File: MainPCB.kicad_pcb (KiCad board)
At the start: 4 copper layers, 105 x 62.4 mm, 57 parts, among them J1 RaspberryPi, J2 Conn_01x05, J3 Screw_Terminal_01x02, J4 Conn_01x02, J5 Conn_01x06, J6 Conn_01x03_Pin, J7 Conn_01x05, J8 Conn_01x12, M1 Motor_DC, M2 Motor_DC, M3 Motor_DC, M4 Motor_DC, M5 Motor_DC, SW1 SW_SPDT, SW2 SW_SPDT, SW3 SW_SPDT, SW4 SW_SPDT, U1 Teensy4.1, U10 Compass, U11 V_Regulator5v, U12 RockerSwitch, U13 V_Regulator3.3v, U2 VNH Driver, U3 VNH Driver, U4 VNH Driver, U5 VNH Driver, U6 TSOP25xx, U7 V_Regulator5v, U8 VNH Driver

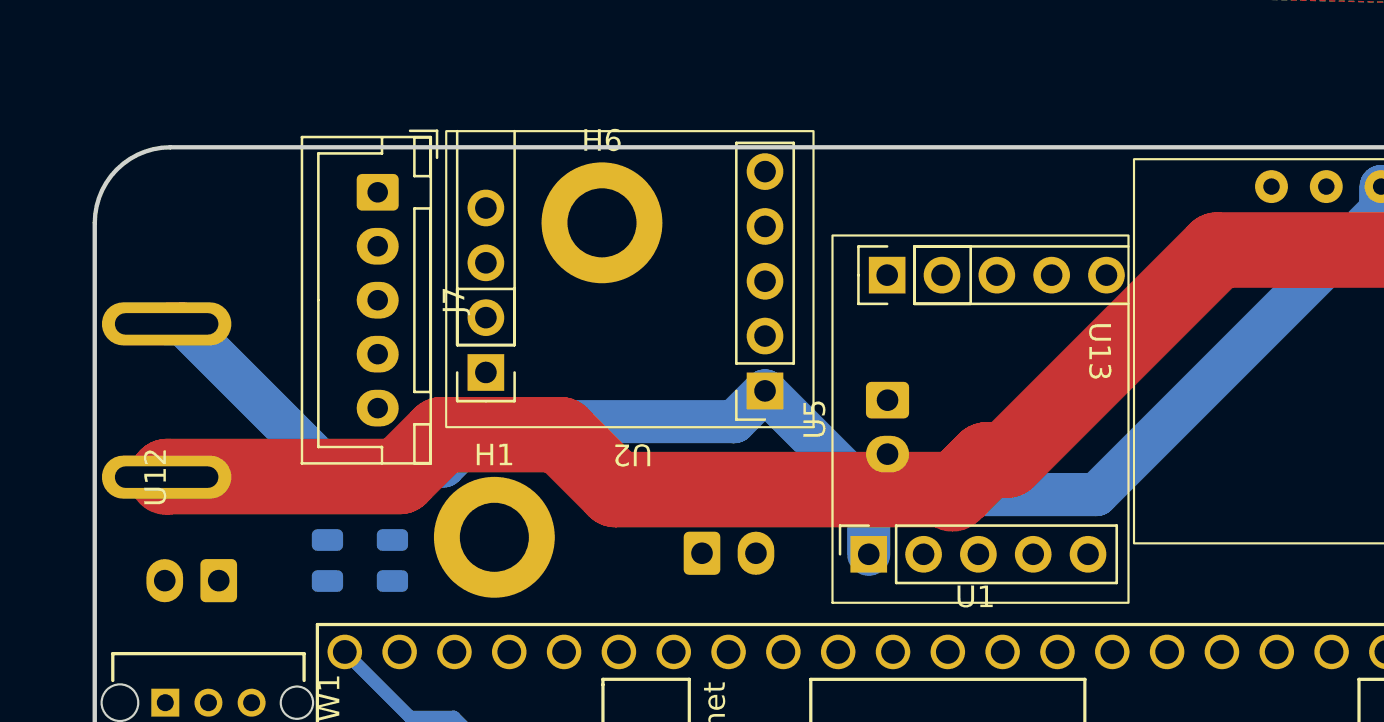
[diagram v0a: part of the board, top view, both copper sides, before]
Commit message: moved stuff
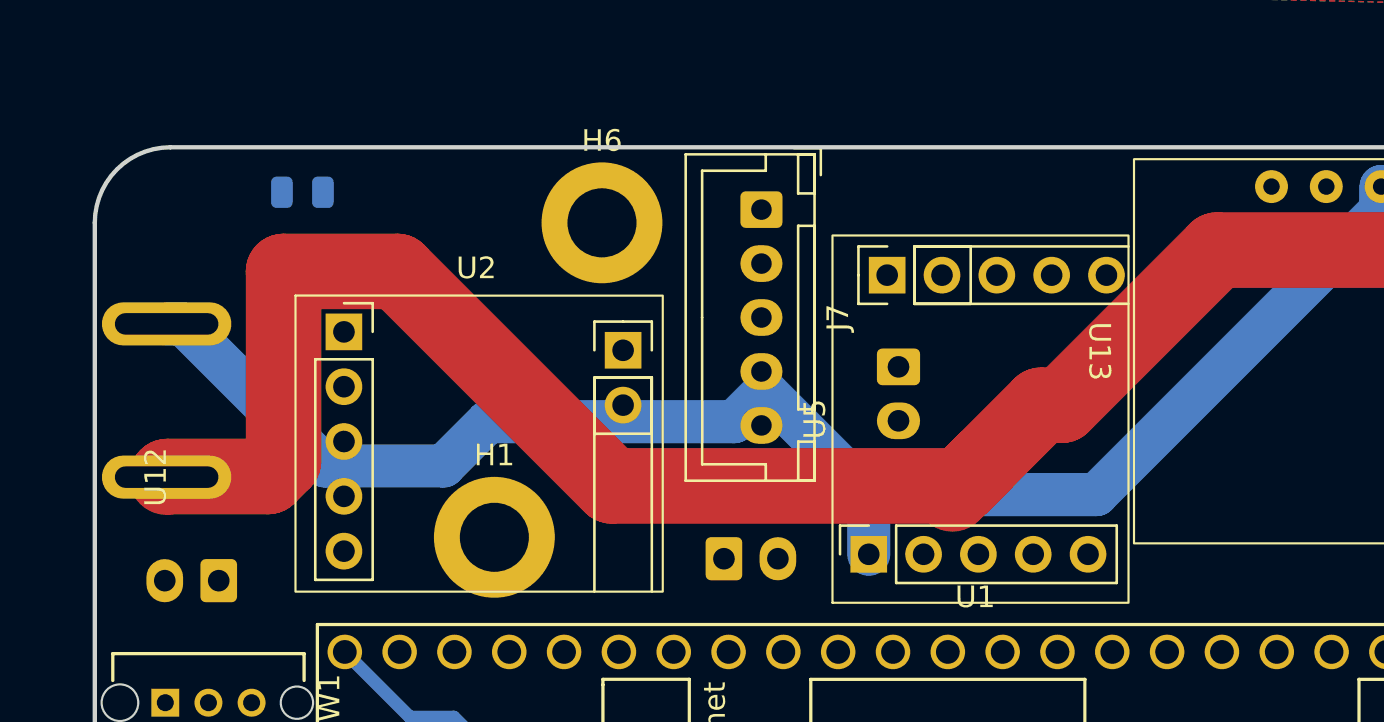
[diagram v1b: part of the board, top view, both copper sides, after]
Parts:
- moved J7 17.8 mm to (118.6, 66.1)
- moved R6 17.6 mm to (97.3, 65.3), turned to 180 degrees
- moved R7 14.1 mm to (97.3, 68.3), turned to 180 degrees
- moved U2 9.80 mm to (105.4, 76.5), turned to 0 degrees
- moved M4 1.63 mm to (125.0, 73.4)
- moved M1 1.05 mm to (116.9, 82.3)
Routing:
- net Net-(J3-Pin_2): track 147.7 -> 159.0 mm
